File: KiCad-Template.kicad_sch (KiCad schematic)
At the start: 1 part, among them U1 ESP32-S3-WROOM-1

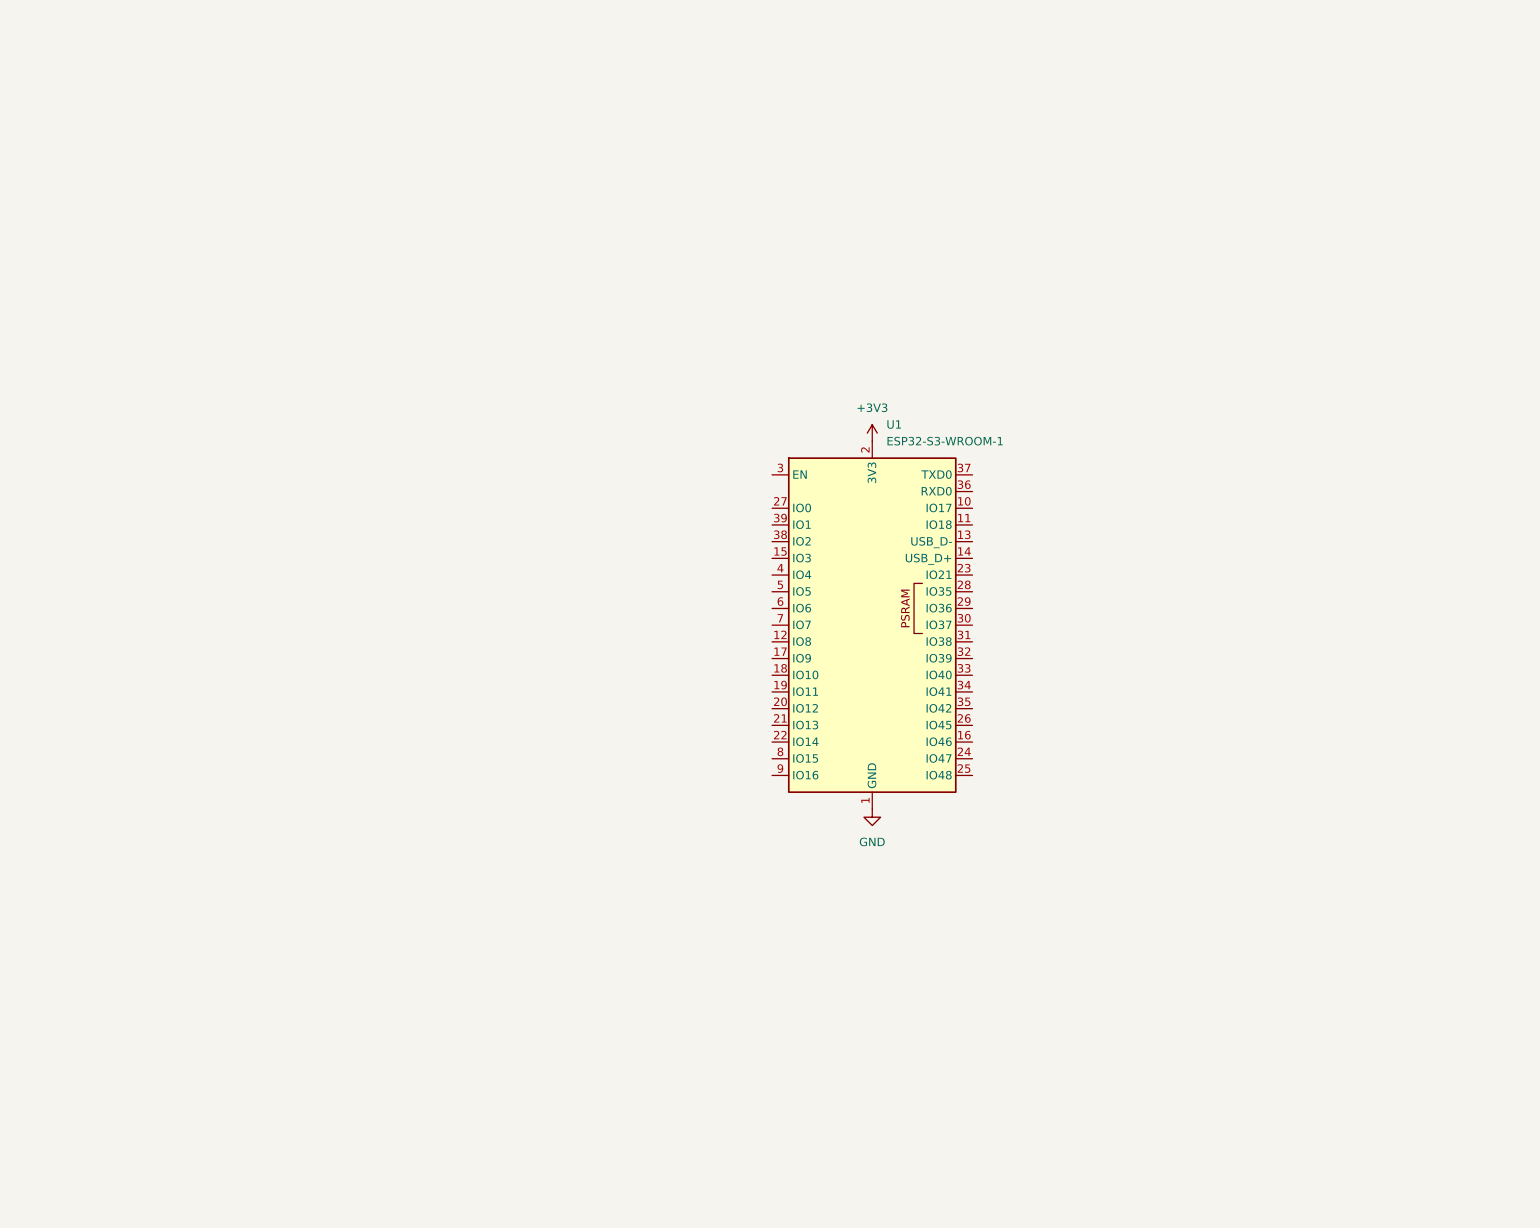
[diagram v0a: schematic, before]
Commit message: Update work sheet
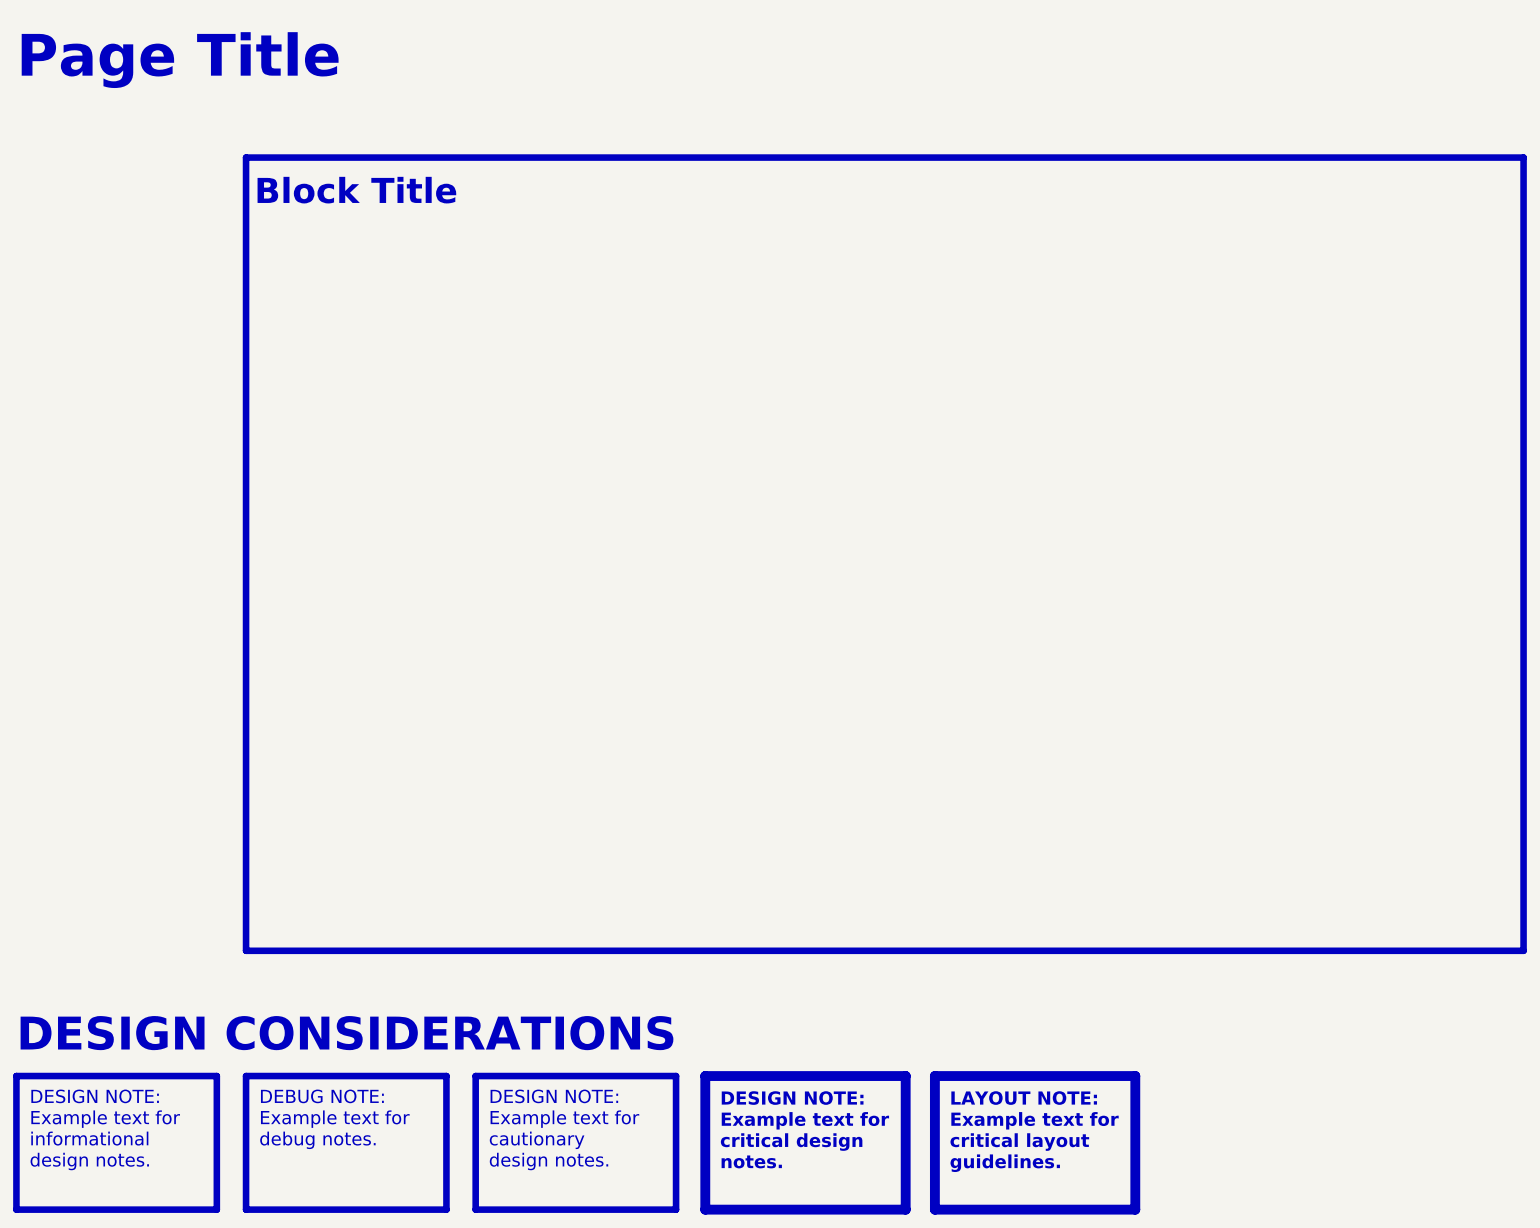
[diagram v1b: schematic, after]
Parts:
- removed U1: ESP32-S3-WROOM-1, Custom:ESP32-S3-WROOM-1, symbol Custom:ESP32-S3-WROOM-1
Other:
- note added: "Block Title"
- note added: "DESIGN CONSIDERATIONS"
- note added: "Page Title"
